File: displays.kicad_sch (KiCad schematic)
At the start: 15 parts, among them J10 LEDX, J11 LEDY, J7 TO-LCD, Q1 2N7002K, Q2 2N7002K, Q3 2N7002K, U8 MAX7221xNG

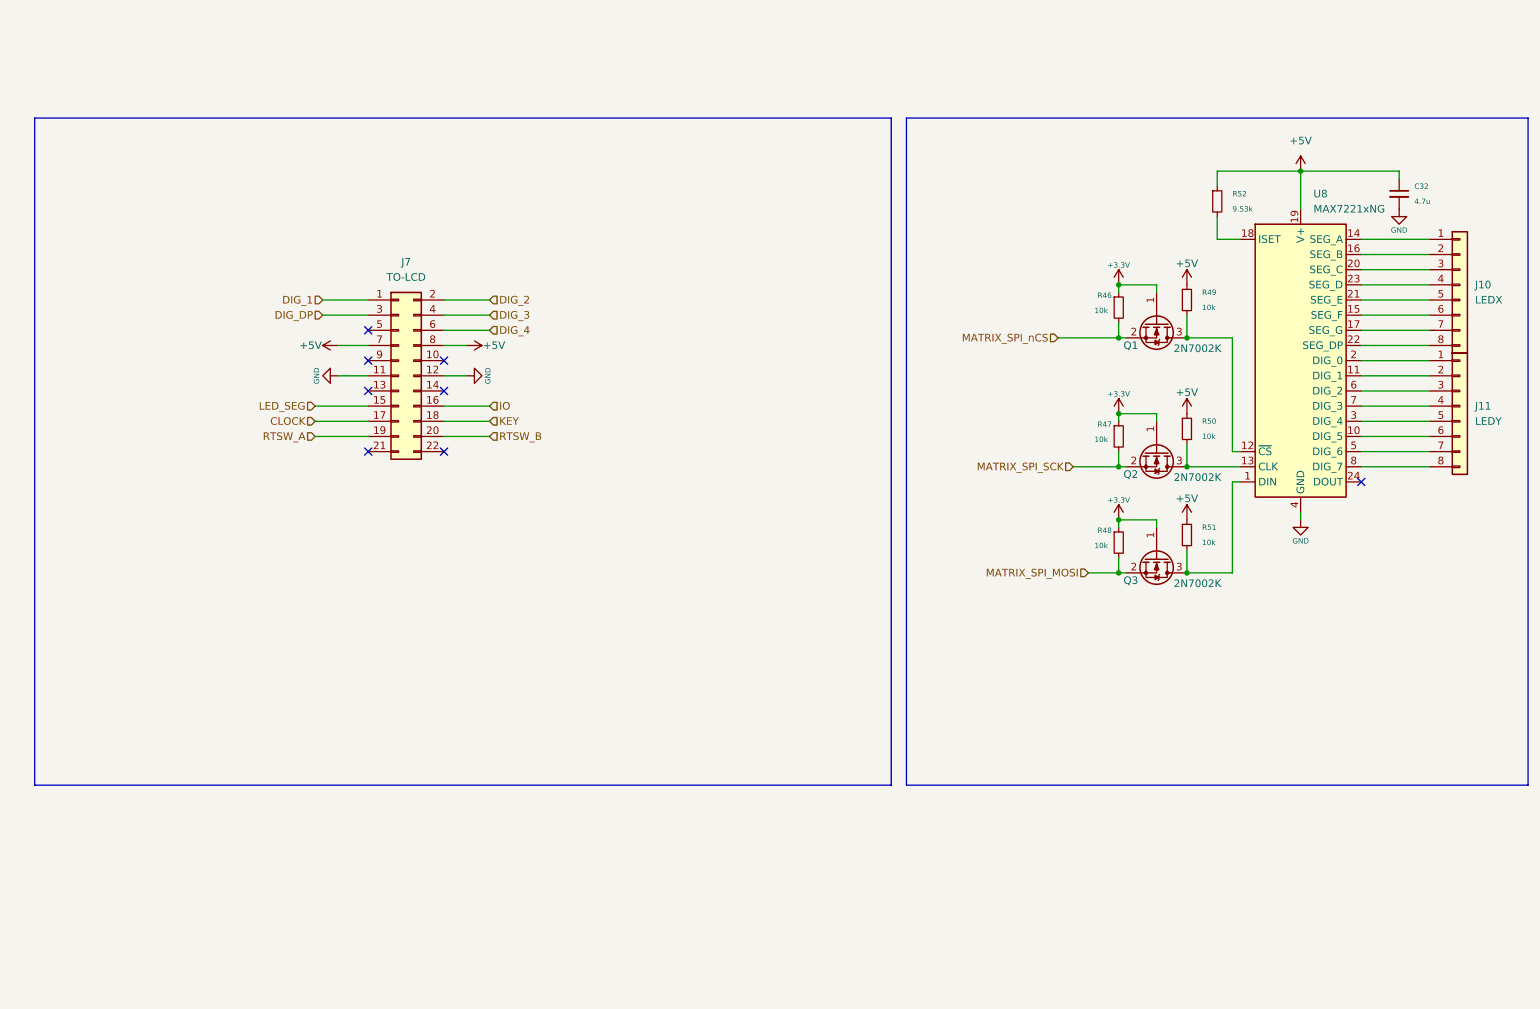
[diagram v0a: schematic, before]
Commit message: Update the source files
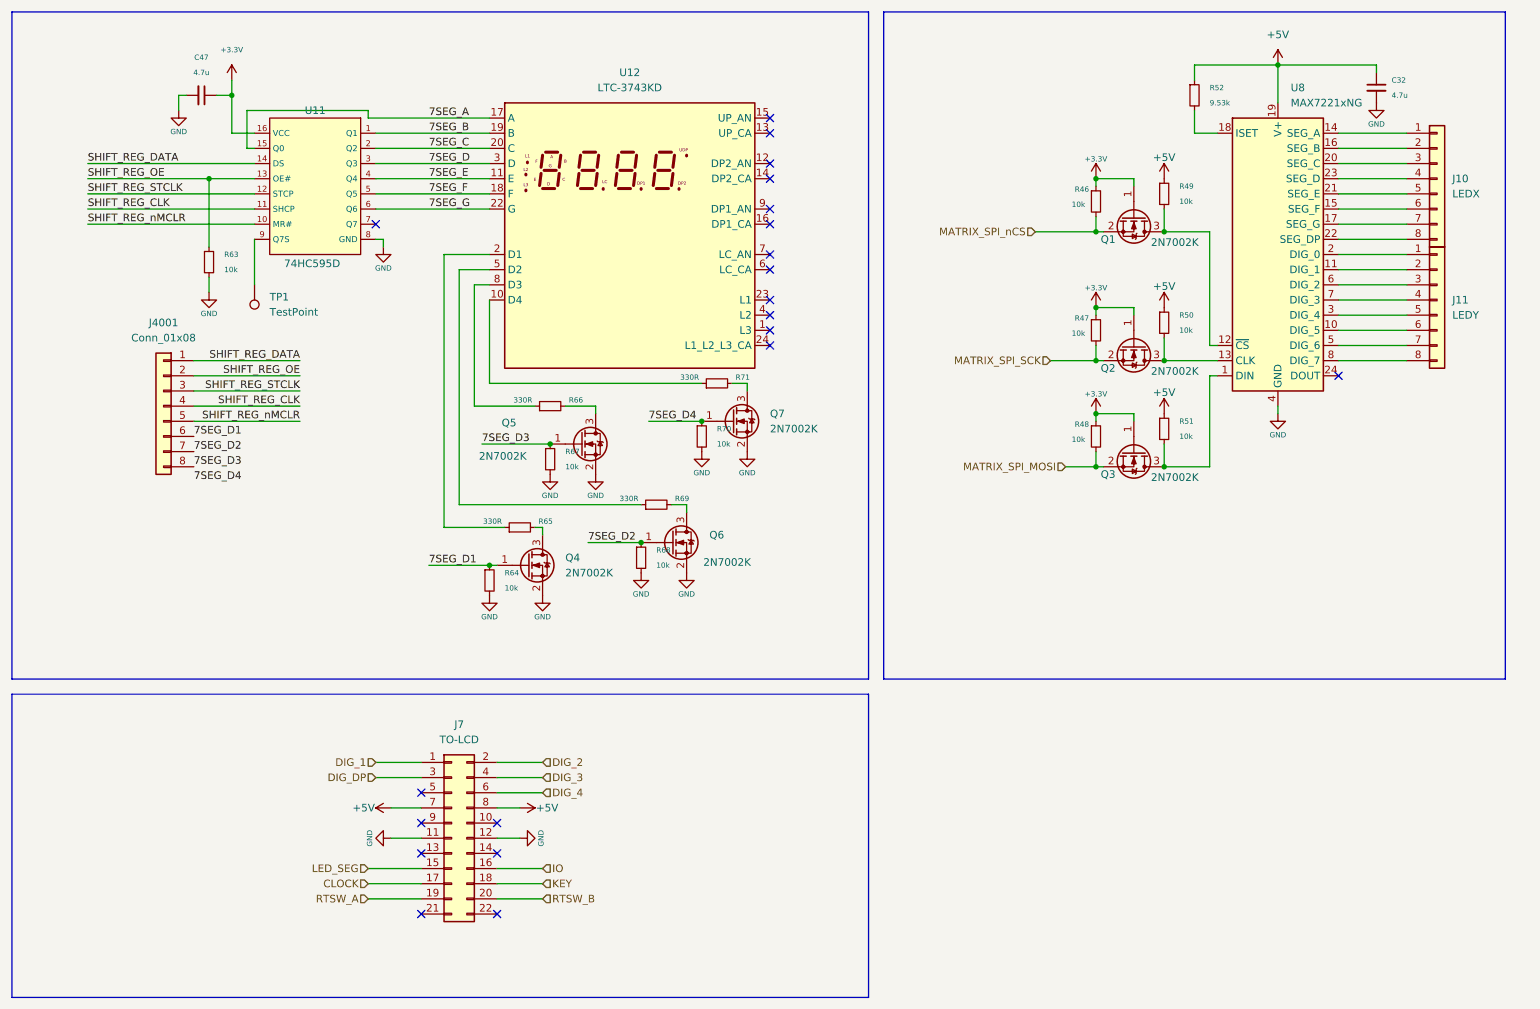
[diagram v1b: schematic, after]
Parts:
- added C47: 4.7u, Capacitor_SMD:C_0603_1608Metric, symbol Device:C_Small
- added J4001: Conn_01x08, Connector_PinSocket_2.54mm:PinSocket_1x08_P2.54mm_Vertical, symbol Connector_Generic:Conn_01x08
- added Q4, Q5, Q6, Q7: 2N7002K, Package_TO_SOT_SMD:SOT-23, symbol Transistor_FET:2N7002K
- added R63, R64, R67, R68, R70: 10k, Resistor_SMD:R_0402_1005Metric, symbol Device:R_Small
- added R65, R66, R69, R71: 330R, Resistor_SMD:R_0402_1005Metric, symbol Device:R_Small
- added TP1: TestPoint, TestPoint:TestPoint_Pad_1.0x1.0mm, symbol Connector:TestPoint
- added U11: 74HC595D, PCM_JLCPCB:SOIC-16_3.9x9.9mm_P1.27mm, symbol PCM_JLCPCB-ICs:Shift Register, 1 In, 8 Out, 74HC595D,118
- added U12: LTC-3743KD, KiCadLocal:LTC-3743KD, symbol KiCadLocal:LTC-3743KD
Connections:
- net +3.3V: now also C47.1, U11.16 (VCC)
- net GND: now also C47.2, Q4.2 (S), Q5.2 (S), Q6.2 (S), Q7.2 (S), R63.2, R64.2, R67.2, R68.2, R70.2, U11.8 (GND)
- new net: TP1.1, U11.9 (Q7S)
- new net: Q5.3 (D), R66.2
- new net: R65.1, U12.2 (D1)
- new net: Q4.3 (D), R65.2
- new net: R71.1, U12.10 (D4)
- new net: R69.1, U12.5 (D2)
- new net: R66.1, U12.8 (D3)
- new net: Q6.3 (D), R69.2
- new net: Q7.3 (D), R71.2
- new net 7SEG_A: U11.15 (Q0), U12.17 (A)
- new net 7SEG_B: U11.1 (Q1), U12.19 (B)
- new net 7SEG_C: U11.2 (Q2), U12.20 (C)
- new net 7SEG_D: U11.3 (Q3), U12.3 (D)
- new net 7SEG_D1: J4001.6 (Pin_6), Q4.1 (G), R64.1
- new net 7SEG_D2: J4001.7 (Pin_7), Q6.1 (G), R68.1
- new net 7SEG_D3: J4001.8 (Pin_8), Q5.1 (G), R67.1
- new net 7SEG_D4: Q7.1 (G), R70.1
- new net 7SEG_E: U11.4 (Q4), U12.11 (E), U12.21 (D1_E_AN)
- new net 7SEG_F: U11.5 (Q5), U12.18 (F)
- new net 7SEG_G: U11.6 (Q6), U12.22 (G)
- new net SHIFT_REG_CLK: J4001.4 (Pin_4), U11.11 (SHCP)
- new net SHIFT_REG_DATA: J4001.1 (Pin_1), U11.14 (DS)
- new net SHIFT_REG_OE: J4001.2 (Pin_2), R63.1, U11.13 (OE#)
- new net SHIFT_REG_STCLK: J4001.3 (Pin_3), U11.12 (STCP)
- new net SHIFT_REG_nMCLR: J4001.5 (Pin_5), U11.10 (MR#)
- no-connect marks 8 -> 21
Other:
- moved on the sheet: C32, J10, J11, J7, Q1, Q2, Q3, R46, R47, R48, R49, R50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
